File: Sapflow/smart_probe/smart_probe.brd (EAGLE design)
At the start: 49.9 x 17.7 mm, 33 parts, among them IC1 MCP3424-E_SL, IC2 PCA9615DPJ

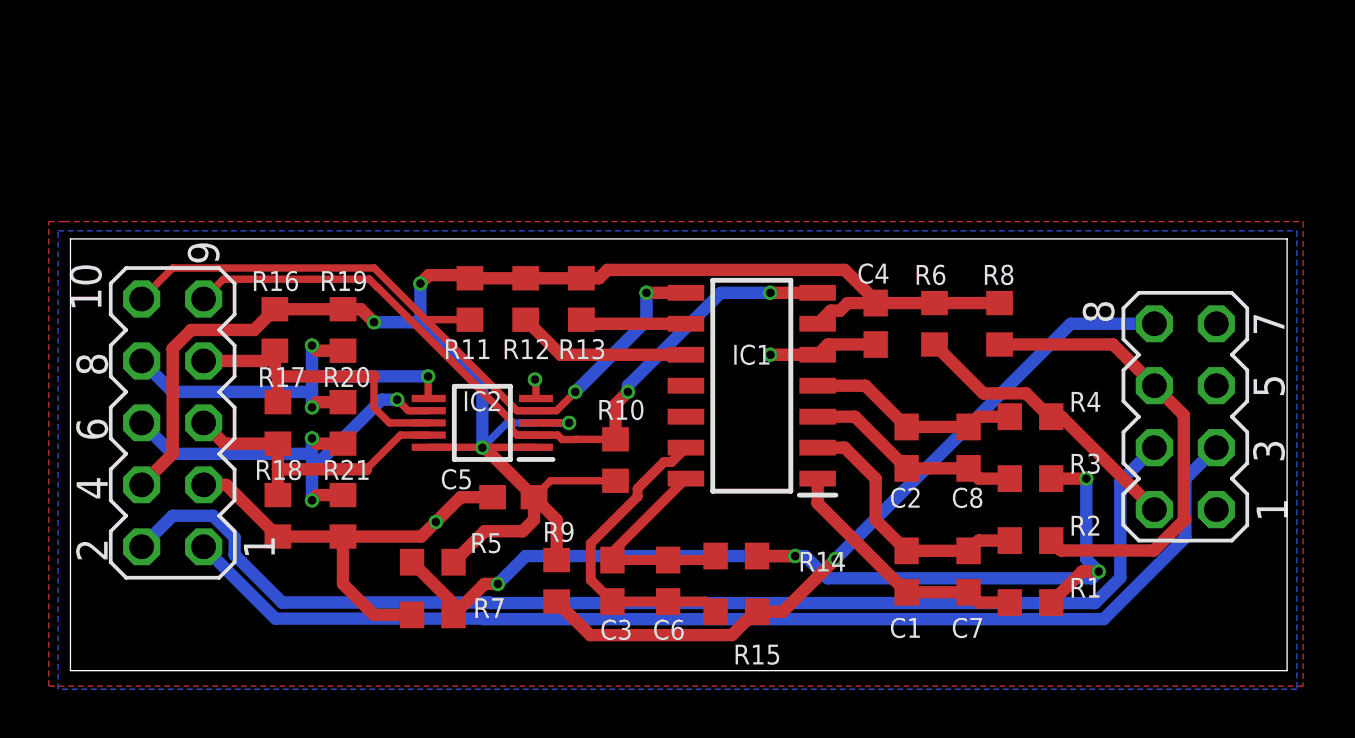
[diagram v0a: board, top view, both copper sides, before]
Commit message: Removed duplicate versions
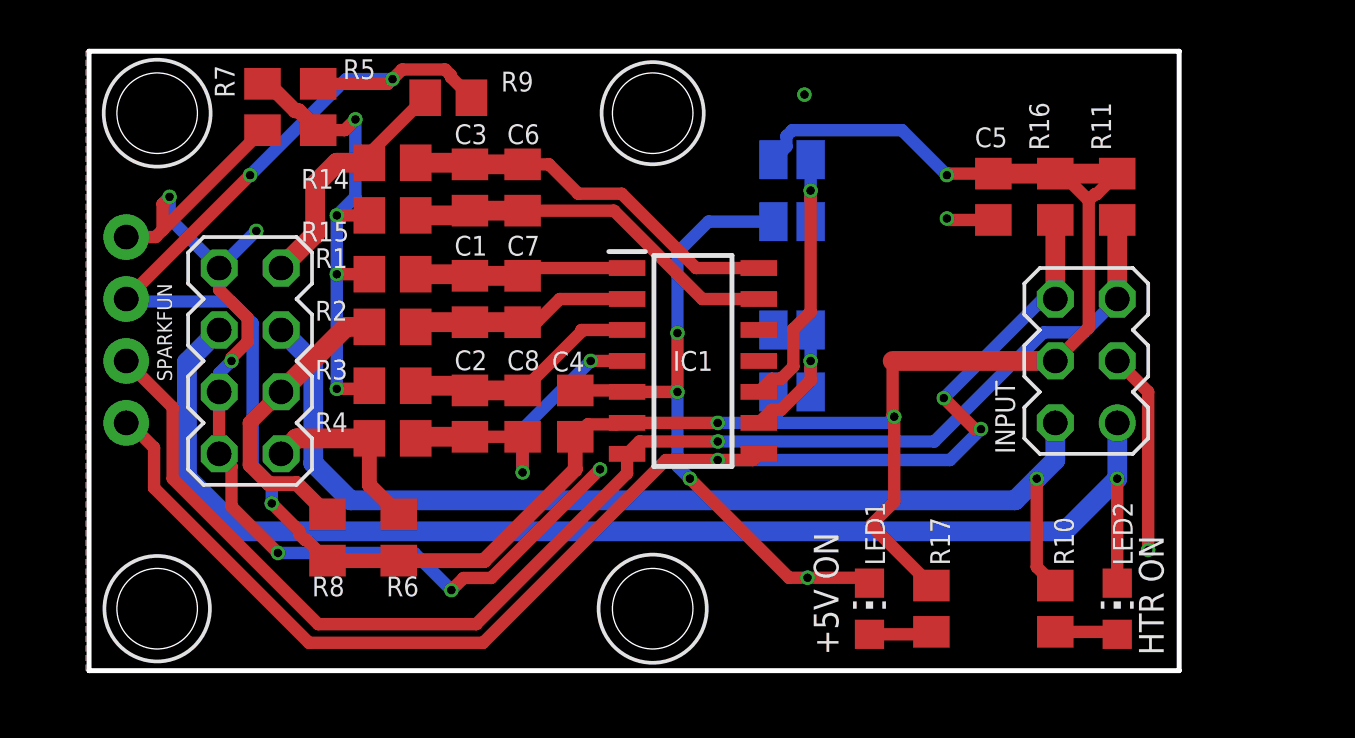
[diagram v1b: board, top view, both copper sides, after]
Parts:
- removed IC2: PCA9615DPJ, PCA9615DPJ:SOP50P490X110-10N
- removed R12, R13: 0, rcl:R0603
- removed R18, R19, R21: 600, rcl:R0603
- removed R20: 120, rcl:R0603
- removed SV1: (no value), con-lstb:MA04-2
- removed SV3: (no value), con-lstb:MA05-2
- added H1, H2, H3, H4: STAND-OFF, SparkFun-Hardware:STAND-OFF
- added INPUT: (no value), better_header:MA03-2
- added LED1, LED2: (no value), led:CHIP-LED0805
- added LOGO1: OSHW-LOGOM, SparkFun-Aesthetics:OSHW-LOGO-M
- added PROBE: (no value), better_header:MA04-2
- added SJ1, SJ2, SJ3, SJ4: (no value), jumper:SJ
- added SPARKFUN: (no value), SparkX:1X04_NO_SILK
- C1, C2, C3, C4, C5, C6, C7, C8: device rcl:C0603 -> rcl:C0805
- R1, R10, R11, R14, R15, R2, R3, R4, R5, R6, R7, R8, R9: device rcl:R0603 -> rcl:R0805
- R16: value 600 -> 5k; device rcl:R0603 -> rcl:R0805
- R17: value 120 -> 1.5k; device rcl:R0603 -> rcl:R0805
- moved R16 32.5 mm to (41.9, 20.7)
- moved R1 29.4 mm to (14.7, 17.5), turned to 0 degrees
- moved R8 28.9 mm to (12.1, 6.73), turned to 270 degrees
- moved R17 27.9 mm to (36.8, 3.81)
- moved R2 27.6 mm to (14.7, 15.4), turned to 0 degrees
- moved R11 26.9 mm to (44.5, 20.7)
- moved R3 26.4 mm to (14.7, 13.0), turned to 0 degrees
- moved R4 26.2 mm to (14.7, 10.8), turned to 0 degrees
- moved R6 23.7 mm to (15.0, 6.73), turned to 270 degrees
- moved C5 23.2 mm to (39.4, 20.7), turned to 270 degrees
- moved R7 22.0 mm to (9.40, 24.4), turned to 90 degrees
- moved R15 21.5 mm to (14.7, 19.9), turned to 180 degrees
- moved C7 21.4 mm to (20.1, 16.5), turned to 270 degrees
- moved R14 21.4 mm to (14.7, 22.1), turned to 180 degrees
- moved C1 21.1 mm to (17.9, 16.5), turned to 270 degrees
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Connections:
- removed net ADR0: IC1.9, R13.1
- removed net ADR1: IC1.10, R12.1
- removed net CLK+: IC2.6, R19.1, R20.2, SV3.8
- removed net CLK-: IC2.7, R20.1, R21.2, SV3.6
- removed net DAT+: IC2.8, R16.1, R17.2, SV3.7
- removed net DAT-: IC2.9, R17.1, R18.2, SV3.5
- new net N$1: LED1.A, R17.1
- new net N$2: LED2.A, R10.1
- new net N$4: IC1.10, SJ1.1, SJ2.1
- new net N$5: IC1.9, SJ3.1, SJ4.1
- net +5V: now also INPUT.4, R17.2, SJ2.2, SJ4.2, SPARKFUN.2; no longer IC2.1, IC2.10, IC2.3, R10.2, R12.2, R13.2, R19.2, SV3.4
- net GND: now also INPUT.3, LED1.C, PROBE.1, PROBE.5, PROBE.7, SJ1.2, SJ3.2, SPARKFUN.1; no longer IC2.5, R18.1, R21.1, SV1.1, SV1.5, SV1.7, SV3.3
- net HTR+: now also INPUT.2, PROBE.4, R10.2; no longer SV1.4, SV3.2
- net HTR-: now also INPUT.1, LED2.C, PROBE.3; no longer SV1.3, SV3.1
- net RTD0+: now also PROBE.8, R4.1, R6.1; no longer R15.2, R9.1, SV1.8
- net RTD1+: now also PROBE.6; no longer SV1.6
- net RTD2+: now also PROBE.2, R14.2, R9.1; no longer R4.1, R6.1, SV1.2
- net SCL(BYPASS): now also INPUT.6, R16.1, SPARKFUN.4; no longer IC2.4, R11.1, SV3.10
- net SDA(BYPASS): now also INPUT.5, R11.1, SPARKFUN.3; no longer IC2.2, R10.1, SV3.9
- net VREF: now also R15.2; no longer R14.2
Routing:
- net GND: track 24.1 -> 81.9 mm, vias 3 -> 13
- net +5V: track 76.6 -> 109.7 mm, vias 4 -> 6
- net SCL(BYPASS): track 29.7 -> 56.7 mm, vias 2 -> 3
- net SDA(BYPASS): track 31.9 -> 56.1 mm, vias 2 -> 1
- net RTD0+: track 30.4 -> 7.50 mm, vias 1 -> 0
- net VREF: track 40.3 -> 20.2 mm
- net CLK-: track 18.9 -> 0.00 mm, vias 3 -> 0
- net CLK+: track 18.4 -> 0.00 mm, vias 3 -> 0
- net DAT+: track 13.0 -> 0.00 mm
- net DAT-: track 12.3 -> 0.00 mm
- net N$4: track 0.00 -> 11.9 mm, vias 0 -> 1
- net ADR1: track 7.17 -> 0.00 mm
- net RTD1+: track 19.3 -> 12.3 mm
- net CH4-: track 8.89 -> 15.9 mm
- net N$5: track 0.00 -> 6.18 mm, vias 0 -> 1
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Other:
- board size 49.9 x 17.7 mm -> 44.7 x 25.4 mm
- board text added: "+5V"
- board text added: "+5V ON"
- board text added: "ADR0"
- board text added: "ADR1"
- board text added: "GND"
- board text added: "HTR ON"
- board text added: "March 2020"
- board text added: "NEVER solder both"
- board text added: "Smart Probe v2.0"
- board text added: "jumpers in a group"
- board text removed: "0.1u"
- board text removed: "1u"
- board text removed: "2"
- board text removed: "3"
- board text removed: "4"
- board text removed: "40k"
- board text removed: "5"
- board text removed: "6"
- board text removed: "7"
- board text removed: "8"
- board text removed: "9"
- board text removed: "DIFF I2C"
- board text removed: "Feb. 2020"
- board text removed: "Smart Probe v1.0"
